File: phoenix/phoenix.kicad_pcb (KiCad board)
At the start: 2 copper layers, 65 x 22.6 mm, 35 parts, among them J1 Ultrafit_2, J2 Micro_SD_Card_Det, J4 Ultrafit_2, J5 Ultrafit_2, P1 CONN_02X03, Q1 IRLML6344, U1 ATMEGA328P-AU, U2 ADX377, U3 MMA8451QT, U4 L6932D1.2, U5 RFTRANS434MHZ, Y1 Crystal_SMD

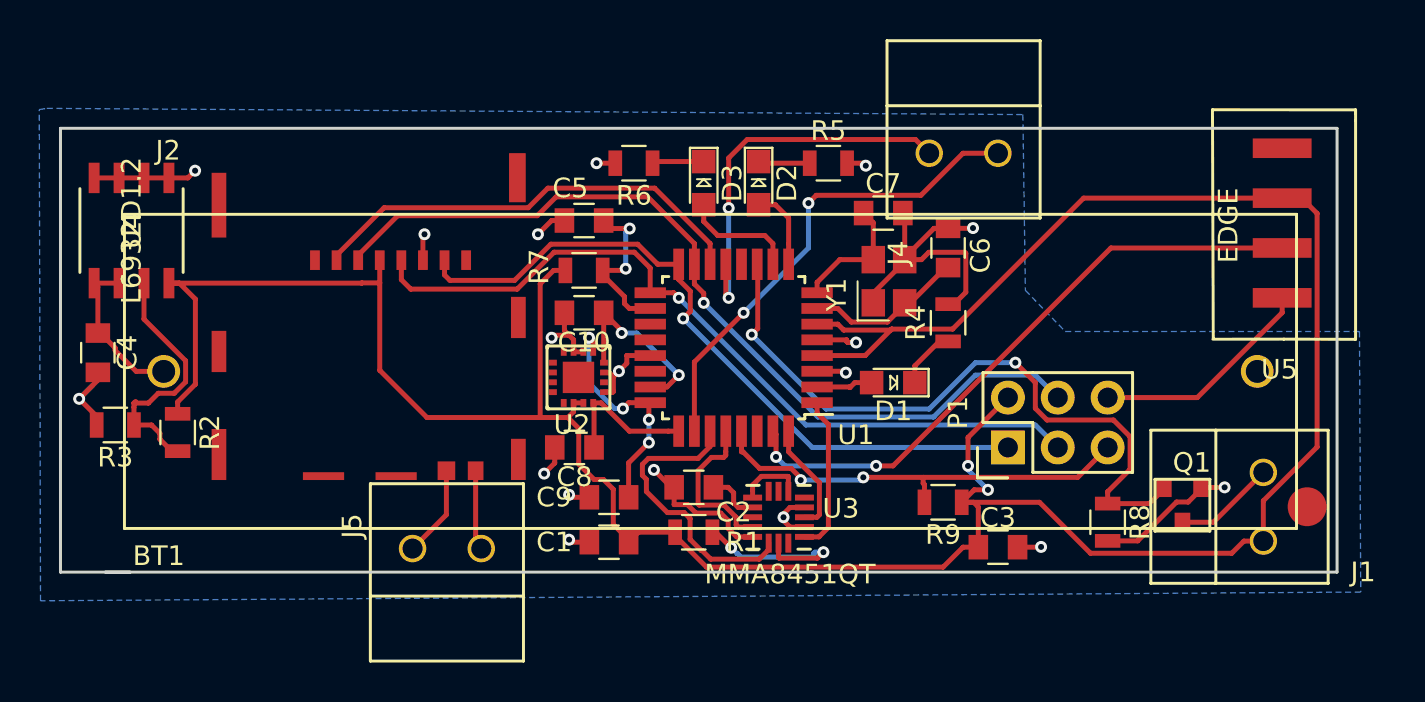
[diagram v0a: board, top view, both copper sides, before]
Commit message: Fix references
stuuf
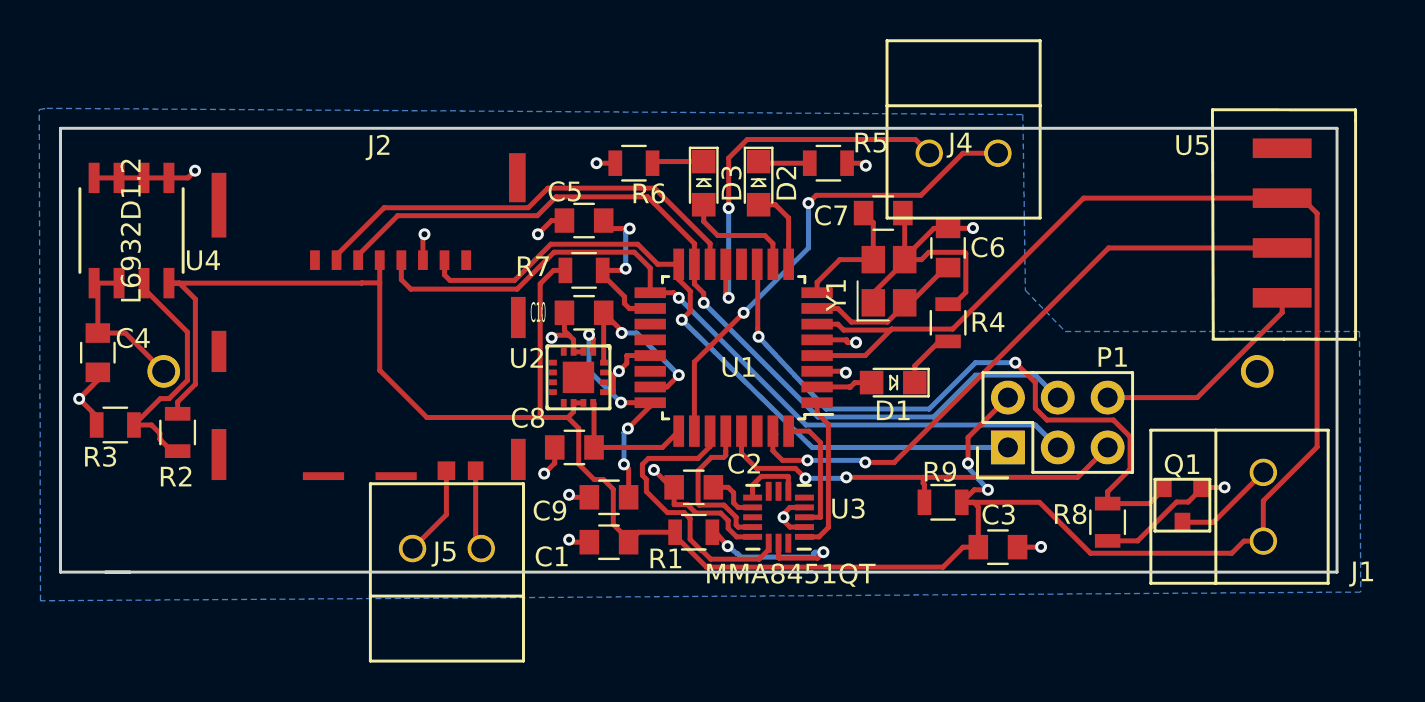
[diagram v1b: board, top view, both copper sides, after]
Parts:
- BT1: moved to B.Cu
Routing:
- net /INT1: track 5.73 -> 6.61 mm
- net Net-(R2-Pad2): track 13.2 -> 12.5 mm
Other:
- board text added: "4/16/18"
- board text added: "Corey Cochran-Lepiz"
- board text added: "ORC"
- board text added: "REV_1"
- board text added: "William Fairman"
